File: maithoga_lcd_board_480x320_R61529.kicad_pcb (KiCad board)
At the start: 2 copper layers, 85 x 54.5 mm, 22 parts, among them P1 Display Connector, P2 LicheePi_Con, P3 TouchXY Connector, U1 TSC2007, U2 DIO5661ST6

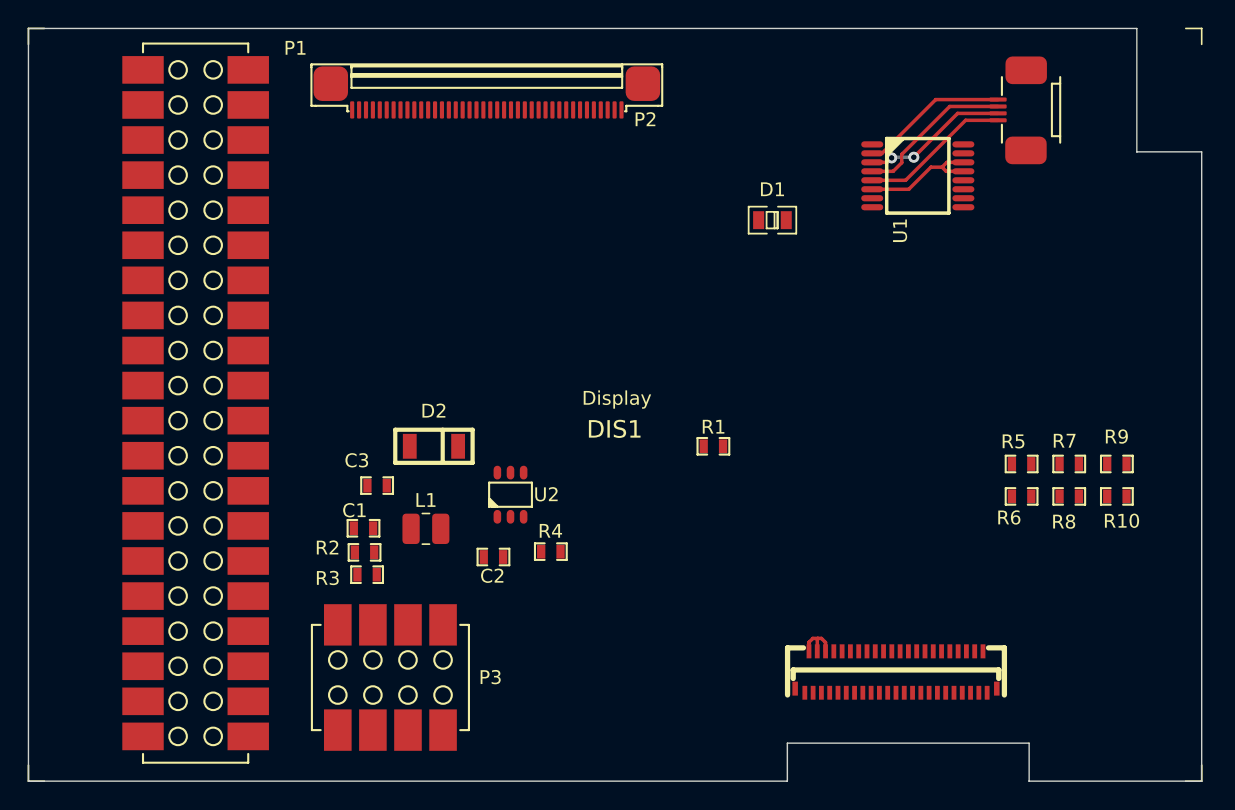
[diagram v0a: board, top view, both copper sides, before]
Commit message: Tracking in progress
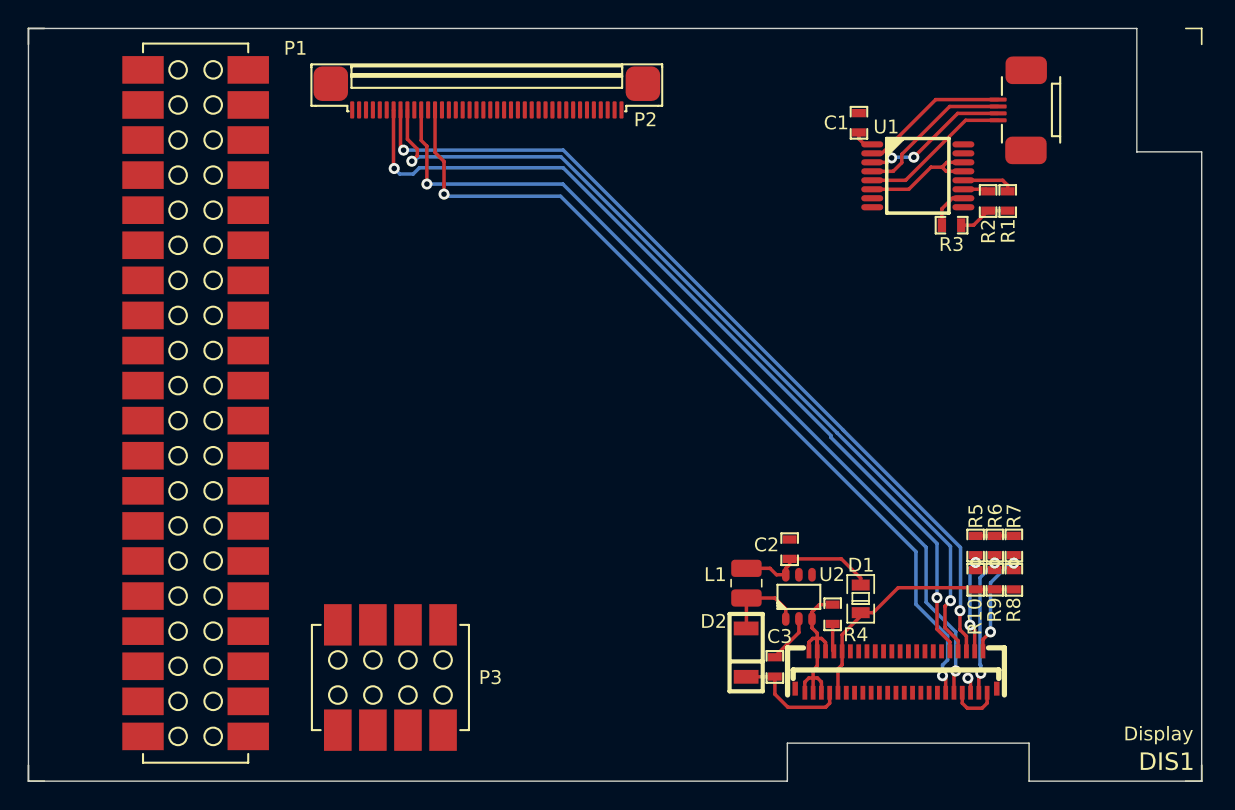
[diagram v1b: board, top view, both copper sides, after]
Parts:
- moved R2 51.8 mm to (171.3, 76.7), turned to 90 degrees
- moved R3 49.3 mm to (168.6, 78.4)
- moved C1 46.4 mm to (161.9, 71.0), turned to 90 degrees
- moved C3 31.7 mm to (155.8, 110.4), turned to 90 degrees
- moved D1 28.2 mm to (162.1, 105.5), turned to 270 degrees
- moved R1 27.7 mm to (172.7, 76.7), turned to 90 degrees
- moved D2 27.1 mm to (153.8, 109.4), turned to 270 degrees
- moved L1 23.5 mm to (153.8, 104.3), turned to 270 degrees
- moved U2 22.2 mm to (157.6, 105.3)
- moved C2 21.5 mm to (156.9, 101.9), turned to 270 degrees
- moved R4 20.9 mm to (160.0, 106.6), turned to 270 degrees
- moved R9 12.2 mm to (171.8, 104.1), turned to 90 degrees
- moved R10 11.9 mm to (170.4, 104.1), turned to 90 degrees
- moved R8 7.25 mm to (173.1, 104.1), turned to 90 degrees
- moved R7 7.14 mm to (173.1, 101.6), turned to 90 degrees
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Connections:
- P3 pad 7: GND -> 3V3
- P3 pad 8: 3V3 -> GND
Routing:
- net /Display and Touchscreen/DISP_DOTCLK: track 0.00 -> 64.1 mm, vias 0 -> 2
- net /Display and Touchscreen/DISP_ENABLE: track 0.00 -> 63.5 mm, vias 0 -> 2
- net /Display and Touchscreen/DISP_HSYNC: track 0.00 -> 63.2 mm, vias 0 -> 2
- net /Display and Touchscreen/DISP_VSYNC: track 0.00 -> 63.0 mm, vias 0 -> 2
- net /Display and Touchscreen/DISP_D17: track 0.00 -> 62.7 mm, vias 0 -> 2
- net Net-(D1-Pad2): track 0.00 -> 18.4 mm
- net 3V3: track 0.00 -> 15.9 mm
- net GND: track 9.08 -> 21.0 mm
- net Net-(DIS1-Pad43): track 0.00 -> 11.0 mm, vias 0 -> 2
- net /Display and Touchscreen/LCD_LED_K: track 3.69 -> 14.6 mm
- net /Display and Touchscreen/LCD_LED_A: track 0.00 -> 8.60 mm
- net Net-(DIS1-Pad44): track 0.00 -> 8.55 mm, vias 0 -> 2
- net Net-(DIS1-Pad42): track 0.00 -> 7.82 mm, vias 0 -> 2
- net Net-(D2-Pad2): track 0.00 -> 6.12 mm
- net /Display and Touchscreen/TOUCHSCREEN_SCL: track 0.00 -> 3.80 mm
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
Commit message: Tracking finished
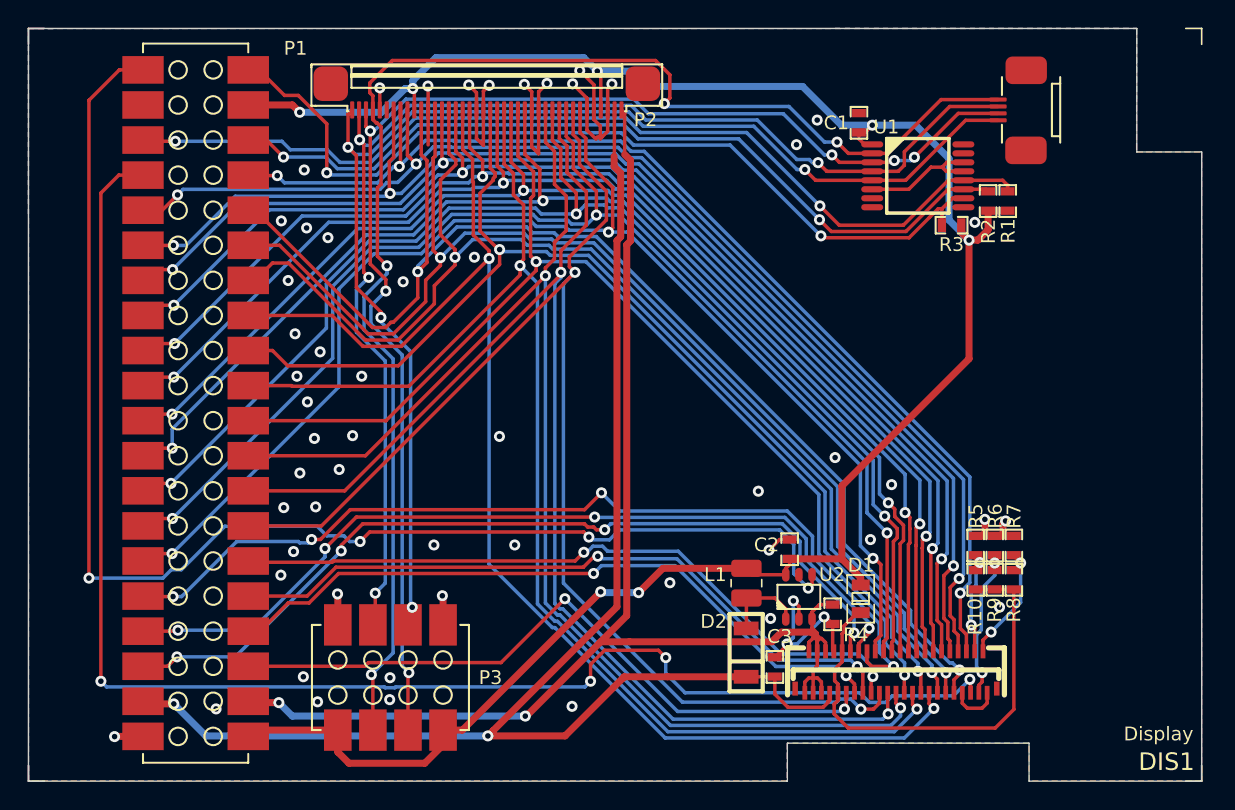
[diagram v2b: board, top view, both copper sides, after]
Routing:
- net 3V3: track 15.9 -> 157.7 mm, vias 0 -> 7
- net /Display and Touchscreen/DISP_~RESET~: track 1.13 -> 107.8 mm, vias 1 -> 4
- net /Display and Touchscreen/BACKLIGHT_PWM: track 0.00 -> 98.4 mm, vias 0 -> 4
- net /Display and Touchscreen/DISP_D0: track 0.00 -> 97.9 mm, vias 0 -> 3
- net /Display and Touchscreen/DISP_D3: track 0.00 -> 96.1 mm, vias 0 -> 2
- net /Display and Touchscreen/DISP_D1: track 0.00 -> 95.9 mm, vias 0 -> 2
- net /Display and Touchscreen/LCD_LED_A: track 8.60 -> 104.5 mm, vias 0 -> 2
- net /Display and Touchscreen/DISP_D2: track 0.00 -> 95.7 mm, vias 0 -> 3
- net /Display and Touchscreen/DISP_D5: track 0.00 -> 95.3 mm, vias 0 -> 2
- net /Display and Touchscreen/DISP_D4: track 0.00 -> 94.3 mm, vias 0 -> 3
- net /Display and Touchscreen/DISP_D13: track 0.00 -> 94.3 mm, vias 0 -> 2
- net /Display and Touchscreen/DISP_D9: track 0.00 -> 94.0 mm, vias 0 -> 2
- net /Display and Touchscreen/DISP_D6: track 0.00 -> 91.6 mm, vias 0 -> 3
- net /Lichee Pi Display Connector/TPX1: track 10.7 -> 102.2 mm, vias 0 -> 4
- net /Display and Touchscreen/DISP_D8: track 0.00 -> 89.8 mm, vias 0 -> 3
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- added copper zone on B.Cu, net GND
- added copper zone on F.Cu, net GND
